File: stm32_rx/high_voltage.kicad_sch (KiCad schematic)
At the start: 12 parts

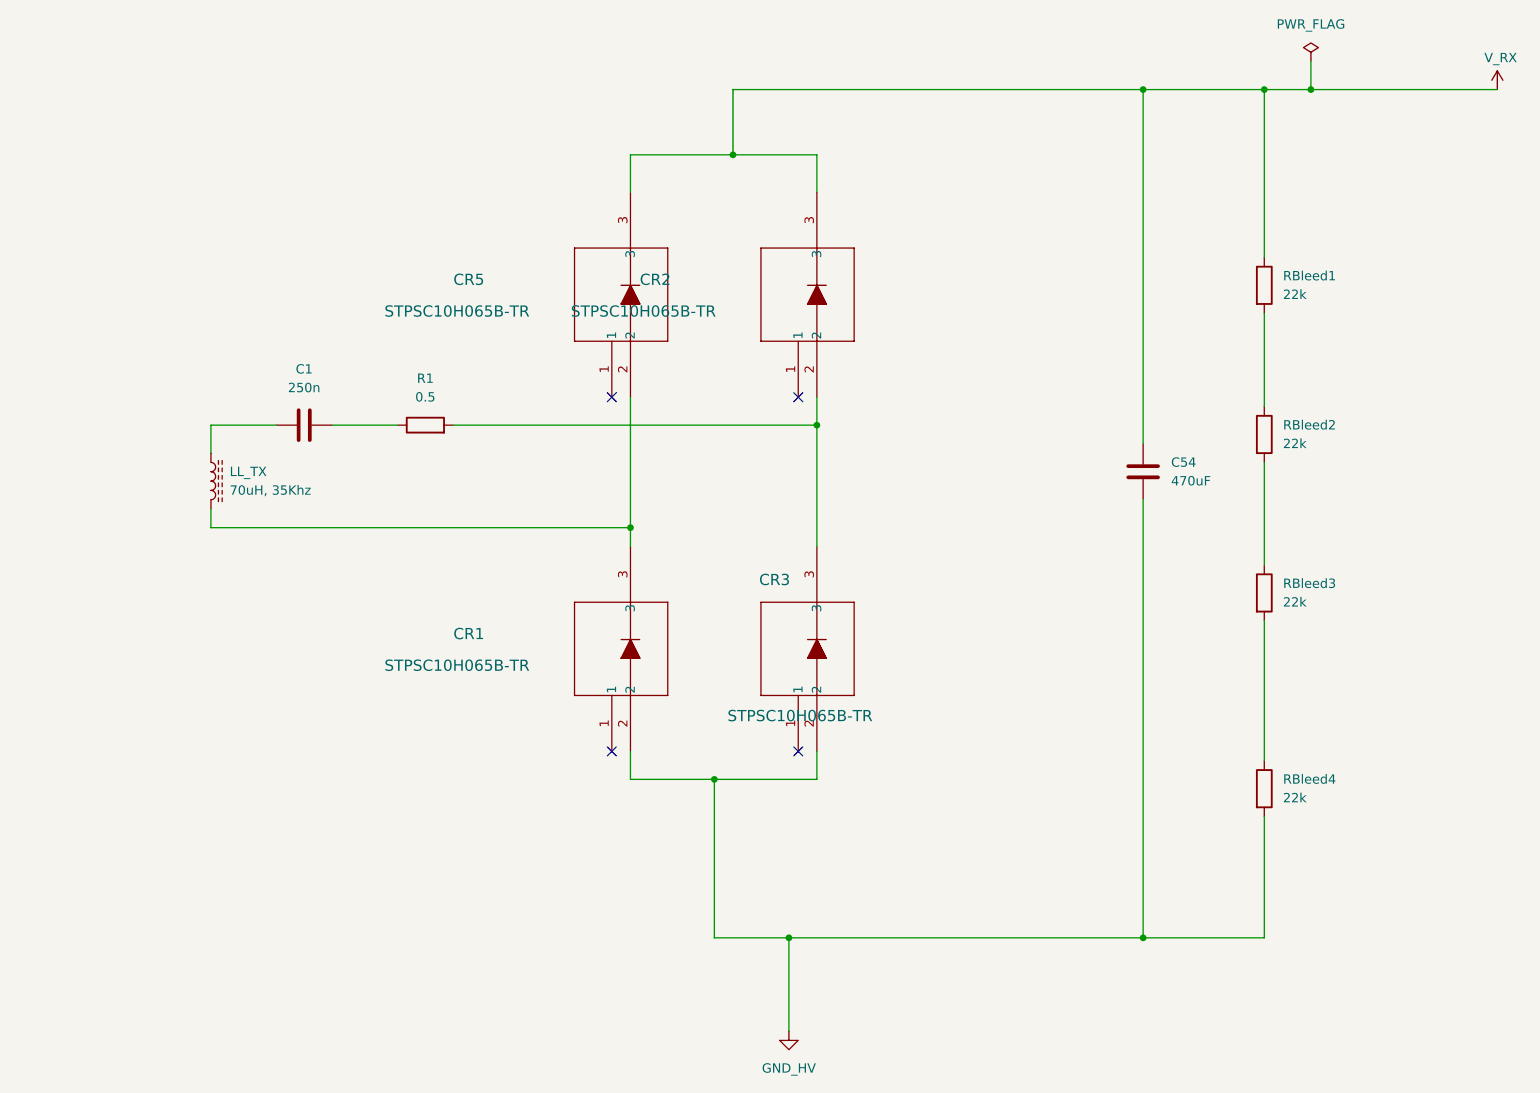
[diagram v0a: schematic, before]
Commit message: Updated file paths in TX project
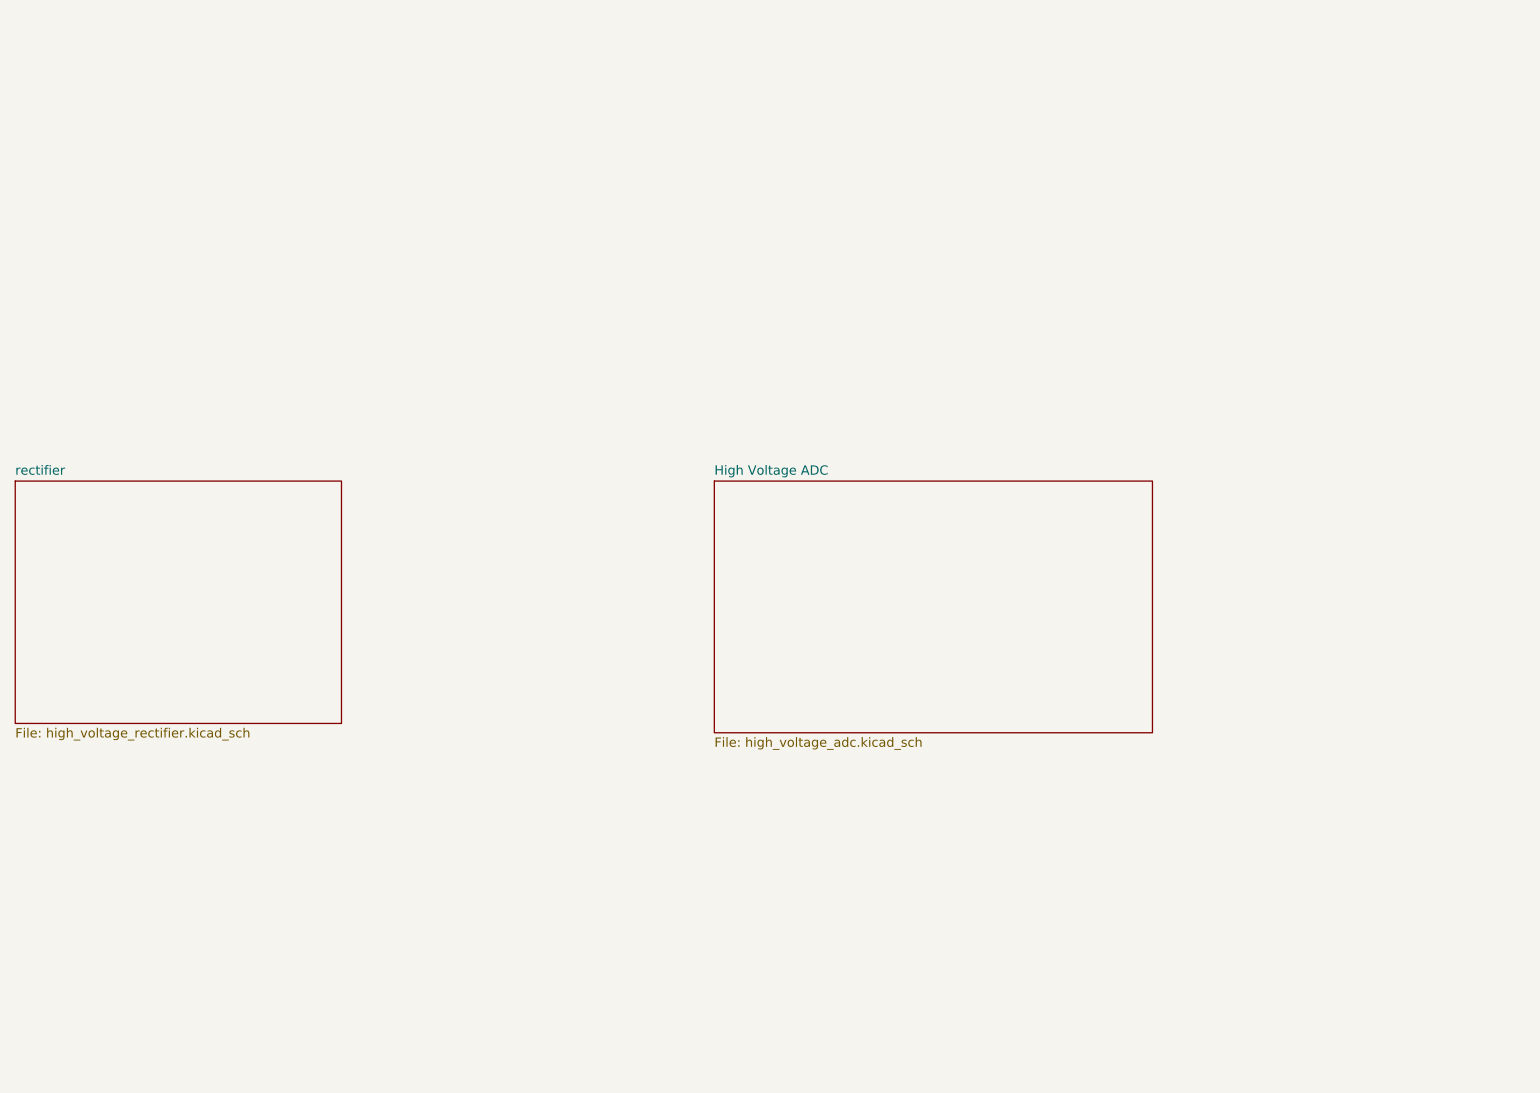
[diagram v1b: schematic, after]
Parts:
- removed C1: 250n, symbol Device:C
- removed C54: 470uF, symbol Device:C
- removed CR1, CR2, CR3, CR5: STPSC10H065B-TR, WPT_TX:DPAK_STPS_STM, symbol 2026-07-24_14-19-21:STPSC10H065B-TR
- removed LL_TX: 70uH, 35Khz, symbol Device:L_Ferrite
- removed R1: 0.5, symbol Device:R
- removed RBleed1, RBleed2, RBleed3, RBleed4: 22k, symbol Device:R
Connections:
- no-connect marks 4 -> 0
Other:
- added sheet High Voltage ADC (high_voltage_adc.kicad_sch)
- added sheet rectifier (high_voltage_rectifier.kicad_sch)
